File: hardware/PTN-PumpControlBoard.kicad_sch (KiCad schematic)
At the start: 33 parts, among them J1 PWR_CAN, J2 Pump_Temp, J3 Flow_Fan, J4 53307-2471, J5 SFH11-PBPC-D05-ST-BK

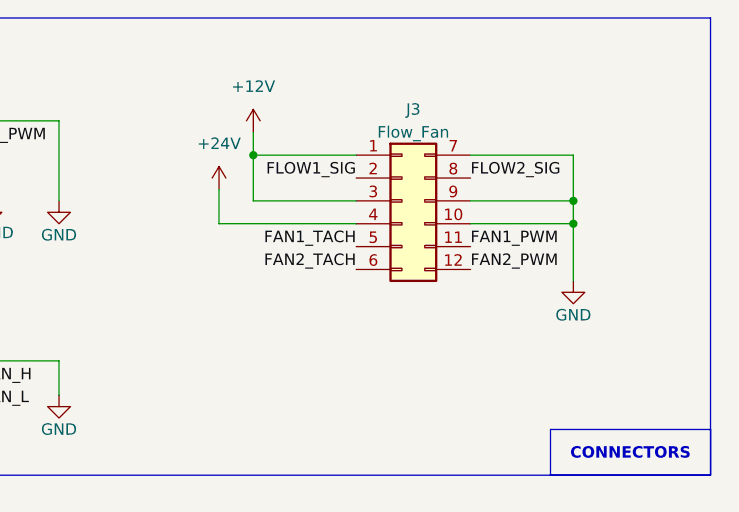
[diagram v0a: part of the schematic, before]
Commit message: Rev c (#4)
* making sure submodules are right

* deleting stuff

* more deletes

* last delete (?)

* hopefully fixed?

* gerbers

* fixed 3d models

* fix .gitignore

Add various entries to .gitignore for build files, Python environments, Mac specific files, Vim swap files, Nix lock files, documentation toolset, and VSCode settings.

* .gitmodules fix

* hopefully firmware setup works?
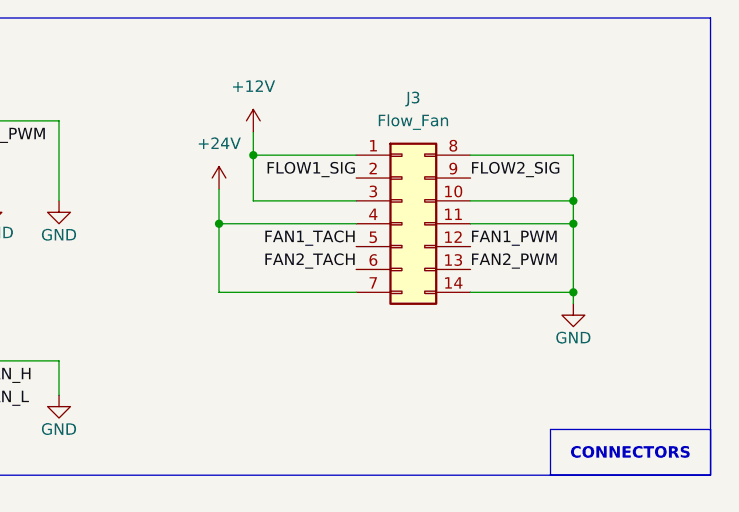
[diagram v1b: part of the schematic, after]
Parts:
- removed J3: Flow_Fan, Connector_Molex:Molex_Nano-Fit_105310-xx12_2x06_P2.50mm_Vertical, symbol Connector_Generic:Conn_02x06_Top_Bottom
- added J3: Flow_Fan, PumpLib:CONN_SD-105310-100_14_MOL, symbol Connector_Generic:Conn_02x07_Top_Bottom
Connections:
- net +12V: now also J3.1 (Pin_1), J3.3 (Pin_3)
- net +24V: now also J3.4 (Pin_4), J3.7 (Pin_7)
- net FAN1_PWM: now also J3.12 (Pin_12)
- net FAN1_TACH: now also J3.5 (Pin_5)
- net FAN2_PWM: now also J3.13 (Pin_13)
- net FAN2_TACH: now also J3.6 (Pin_6)
- net FLOW1_SIG: now also J3.2 (Pin_2)
- net FLOW2_SIG: now also J3.9 (Pin_9)
- net GND: now also J3.10 (Pin_10), J3.11 (Pin_11), J3.14 (Pin_14), J3.8 (Pin_8)
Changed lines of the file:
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@@
 	)
 	(junction
+		(at 259.08 45.72)
+		(diameter 0)
+		(color 0 0 0 0)
+	)
+	(junction
 		(at 90.17 85.09)
 		(diameter 0)
@@
 	)
 	(junction
+		(at 219.71 38.1)
+		(diameter 0)
+		(color 0 0 0 0)
+	)
+	(junction
 		(at 223.52 30.48)
 		(diameter 0)
@@
 	(wire
 		(pts
+			(xy 247.65 45.72) (xy 259.08 45.72)
+		)
+		(stroke
+			(width 0)
+			(type default)
+		)
+	)
+	(wire
+		(pts
 			(xy 27.94 69.85) (xy 29.21 69.85)
 		)
@@
 	(wire
 		(pts
+			(xy 219.71 45.72) (xy 219.71 38.1)
+		)
+		(stroke
+			(width 0)
+			(type default)
+		)
+	)
+	(wire
+		(pts
 			(xy 90.17 82.55) (xy 90.17 85.09)
 		)
@@
 	(wire
 		(pts
+			(xy 259.08 45.72) (xy 259.08 46.99)
+		)
+		(stroke
+			(width 0)
+			(type default)
+		)
+	)
+	(wire
+		(pts
 			(xy 90.17 33.02) (xy 90.17 34.29)
 		)
@@
 	(wire
 		(pts
+			(xy 234.95 45.72) (xy 219.71 45.72)
+		)
+		(stroke
+			(width 0)
+			(type default)
+		)
+	)
+	(wire
+		(pts
 			(xy 130.81 34.29) (xy 130.81 33.02)
 		)
@@
 	(wire
 		(pts
-			(xy 259.08 38.1) (xy 259.08 44.45)
+			(xy 259.08 38.1) (xy 259.08 45.72)
 		)
 		(stroke
@@
 	)
 	(symbol
-		(lib_id "Connector_Generic:Conn_02x06_Top_Bottom")
-		(at 240.03 35.56 0)
-		(unit 1)
-		(exclude_from_sim no)
-		(in_bom yes)
-		(on_board yes)
-		(dnp no)
-		(fields_autoplaced yes)
-		(property "Reference" "J3"
-			(at 241.3 25.4 0)
-			(effects
-				(font
-					(size 1.27 1.27)
-				)
-			)
-		)
-		(property "Value" "Flow_Fan"
-			(at 241.3 27.94 0)
-			(effects
-				(font
-					(size 1.27 1.27)
-				)
-			)
-		)
-		(property "Footprint" "Connector_Molex:Molex_Nano-Fit_105310-xx12_2x06_P2.50mm_Vertical"
-			(at 240.03 35.56 0)
-			(effects
-				(font
-					(size 1.27 1.27)
-				)
-				(hide yes)
-			)
-		)
-		(property "Datasheet" "~"
-			(at 240.03 35.56 0)
-			(effects
-				(font
-					(size 1.27 1.27)
-				)
-				(hide yes)
-			)
-		)
-		(property "Description" "Generic connector, double row, 02x06, top/bottom pin numbering scheme (row 1: 1...pins_per_row, row2: pins_per_row+1 ... num_pins), script generated (kicad-library-utils/schlib/autogen/connector/)"
-			(at 240.03 35.56 0)
-			(effects
-				(font
-					(size 1.27 1.27)
-				)
-				(hide yes)
-			)
-		)
-		(pin "11"
-		)
-		(pin "12"
-		)
-		(pin "6"
-		)
-		(pin "8"
-		)
-		(pin "7"
-		)
-		(pin "10"
-		)
-		(pin "9"
-		)
-		(pin "3"
-		)
-		(pin "5"
-		)
-		(pin "1"
-		)
-		(pin "2"
-		)
-		(pin "4"
-		)
-		(instances
-			(project ""
-				(path "/591f46f8-eb1d-42dc-a4cb-8182eac4ef58"
-					(reference "J3")
-					(unit 1)
-				)
-			)
-		)
-	)
-	(symbol
 		(lib_id "power:GND")
-		(at 259.08 44.45 0)
+		(at 259.08 46.99 0)
 		(unit 1)
 		(exclude_from_sim no)
@@
 		(dnp no)
 		(property "Reference" "#PWR039"
-			(at 259.08 50.8 0)
+			(at 259.08 53.34 0)
 			(effects
 				(font
@@
 		)
 		(property "Value" "GND"
-			(at 259.08 48.26 0)
+			(at 259.08 50.8 0)
 			(effects
 				(font
@@
 		)
 		(property "Footprint" ""
-			(at 259.08 44.45 0)
+			(at 259.08 46.99 0)
 			(effects
 				(font
@@
 		)
 		(property "Datasheet" ""
-			(at 259.08 44.45 0)
+			(at 259.08 46.99 0)
 			(effects
 				(font
@@
 		)
 		(property "Description" "Power symbol creates a global label with name \"GND\" , ground"
-			(at 259.08 44.45 0)
+			(at 259.08 46.99 0)
 			(effects
 				(font
@@
 					(unit 1)
 				)
+			)
+		)
+	)
+	(symbol
+		(lib_id "Connector_Generic:Conn_02x07_Top_Bottom")
+		(at 240.03 38.1 0)
+		(unit 1)
+		(exclude_from_sim no)
+		(in_bom yes)
+		(on_board yes)
+		(dnp no)
+		(fields_autoplaced yes)
+		(property "Reference" "J3"
+			(at 241.3 24.13 0)
+			(effects
+				(font
+					(size 1.27 1.27)
+				)
+			)
+		)
+		(property "Value" "Flow_Fan"
+			(at 241.3 26.67 0)
+			(effects
+				(font
+					(size 1.27 1.27)
+				)
+			)
+		)
+		(property "Footprint" "PumpLib:CONN_SD-105310-100_14_MOL"
+			(at 240.03 38.1 0)
+			(effects
+				(font
+					(size 1.27 1.27)
+				)
+				(hide yes)
+			)
+		)
+		(property "Datasheet" "~"
+			(at 240.03 38.1 0)
+			(effects
+				(font
+					(size 1.27 1.27)
+				)
+				(hide yes)
+			)
+		)
+		(property "Description" "Generic connector, double row, 02x07, top/bottom pin numbering scheme (row 1: 1...pins_per_row, row2: pins_per_row+1 ... num_pins), script generated (kicad-library-utils/schlib/autogen/connector/)"
+			(at 240.03 38.1 0)
+			(effects
+				(font
+					(size 1.27 1.27)
+				)
+				(hide yes)
+			)
+		)
+		(pin "2"
+		)
+		(pin "3"
+		)
+		(pin "4"
+		)
+		(pin "5"
+		)
+		(pin "6"
+		)
+		(pin "7"
+		)
+		(pin "8"
+		)
+		(pin "9"
+		)
+		(pin "10"
+		)
+		(pin "11"
+		)
+		(pin "12"
+		)
+		(pin "13"
+		)
+		(pin "14"
+		)
+		(pin "1"
+		)
+		(instances
+			(project ""
+				(path "/591f46f8-eb1d-42dc-a4cb-8182eac4ef58"
+					(reference "J3")
+					(unit 1)
+				)
